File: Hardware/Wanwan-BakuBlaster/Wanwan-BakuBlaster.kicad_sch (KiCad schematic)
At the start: 69 parts, among them Q1 BSS138, U1 RP2040-Zero, U2 PT8211, U3 TLV2372

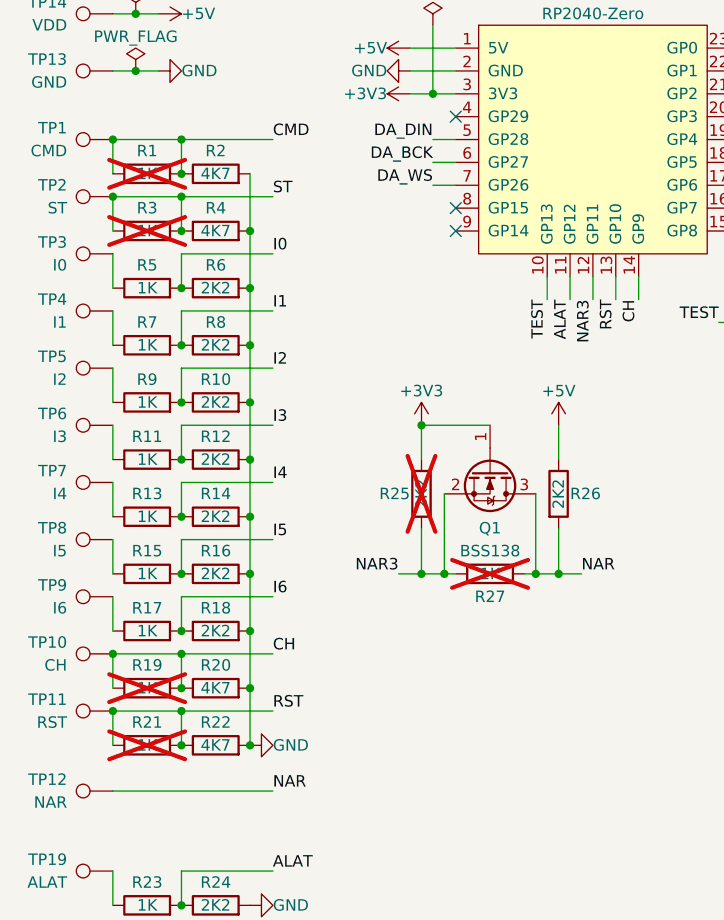
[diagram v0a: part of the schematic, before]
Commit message: Update hardware stuff
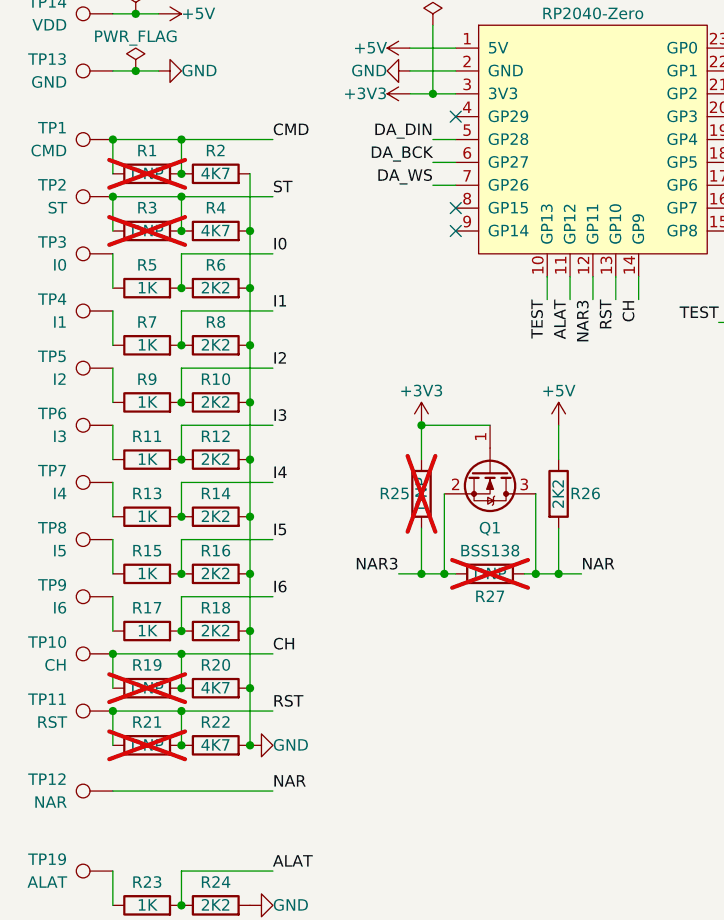
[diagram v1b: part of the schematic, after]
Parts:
- R1, R19, R21, R27, R3: value 1K -> DNP
- R25: value 2K2 -> DNP
